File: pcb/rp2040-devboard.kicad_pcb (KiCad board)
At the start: 2 copper layers, 37.8 x 62.5 mm, 35 parts, among them J201 USB_C_Receptacle_USB2.0_16P, J601 Conn_01x20, J602 Conn_01x20, J603 Conn_01x03, SW401 SW_Push, SW501 SW_Push, U301 TC1017-xLT, U401 RP2040, U501 W25Q128JVS, Y401 ABM8-272-T3

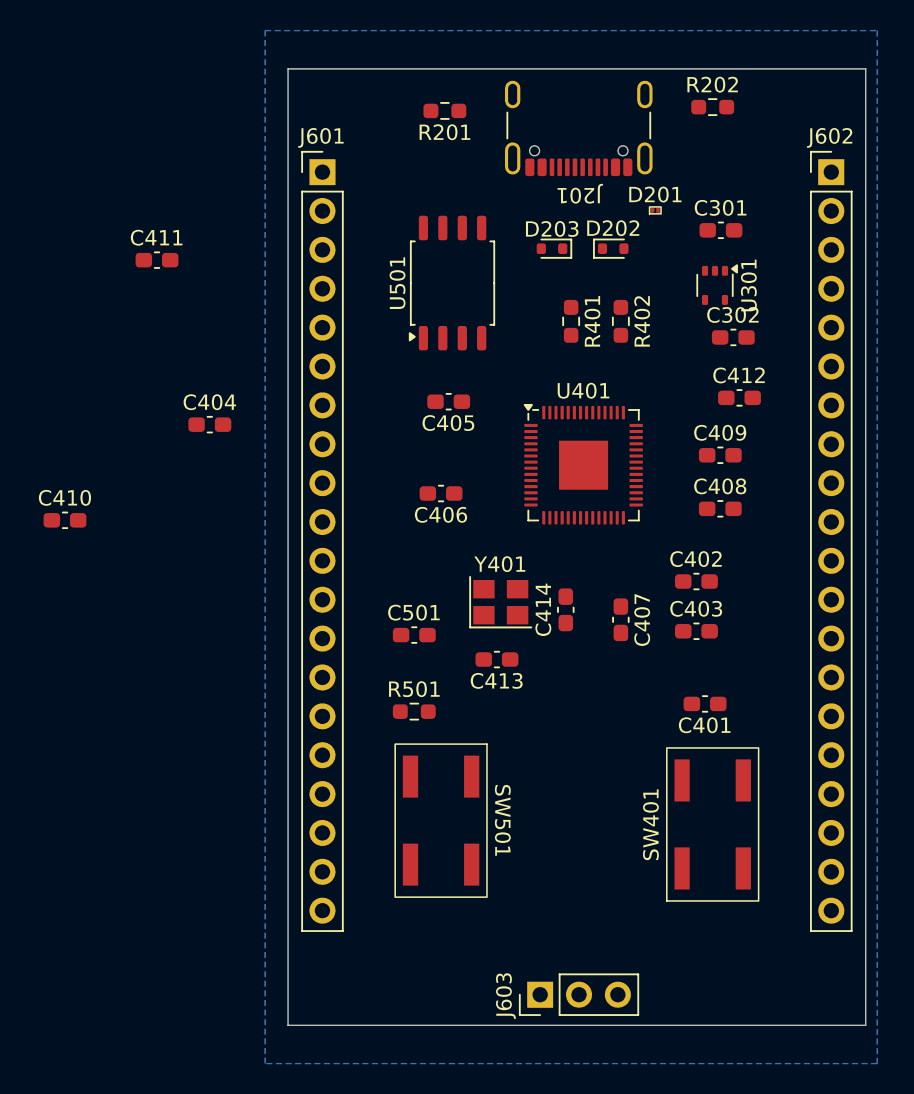
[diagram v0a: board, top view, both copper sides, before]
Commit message: wip pcb placement
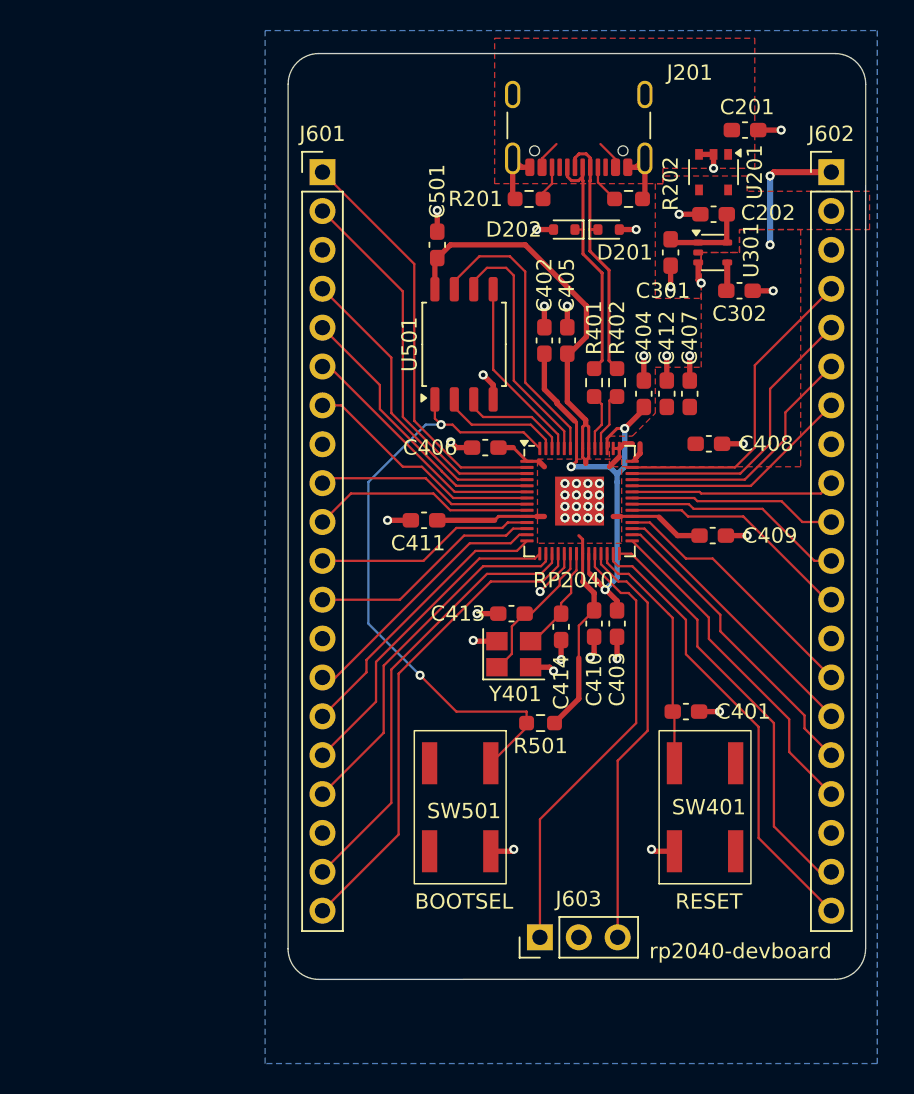
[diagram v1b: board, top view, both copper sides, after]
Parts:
- removed the D201 at (163.0, 56.8)
- added C201: 1u, Capacitor_SMD:C_0603_1608Metric_Pad1.08x0.95mm_HandSolder, F.Cu at (168.9, 51.5)
- added C202: 1u, Capacitor_SMD:C_0603_1608Metric_Pad1.08x0.95mm_HandSolder, F.Cu at (166.8, 57.0)
- added U201: NCP360SN, Package_SO:TSOP-5_1.65x3.05mm_P0.95mm, F.Cu at (166.8, 54.2)
- moved C410 35.2 mm to (159.0, 83.8), turned to -90 degrees
- moved C404 28.4 mm to (162.2, 68.7), turned to 90 degrees
- moved C501 25.5 mm to (148.8, 59.0), turned to 90 degrees
- moved C411 24.4 mm to (147.9, 77.0), turned to 180 degrees
- moved C402 18.6 mm to (155.8, 65.2), turned to 90 degrees
- moved C407 15.4 mm to (165.2, 68.7), turned to 90 degrees
- moved C405 8.72 mm to (157.2, 65.2), turned to 90 degrees
- moved R501 8.28 mm to (155.5, 90.2), turned to 180 degrees
- moved R202 8.14 mm to (161.2, 56.0)
- moved R201 7.96 mm to (154.8, 56.0)
- moved C409 5.27 mm to (166.8, 78.0)
- moved C403 5.21 mm to (160.5, 83.8), turned to -90 degrees
- moved C412 4.76 mm to (163.8, 68.7), turned to 90 degrees
- moved C408 4.32 mm to (166.5, 72.0)
- moved R401 4.27 mm to (159.0, 68.0)
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- renumbered D202 to D201, D203 to D202
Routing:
- net +3V3: track 0.00 -> 73.1 mm, vias 0 -> 2
- net GND: track 0.00 -> 52.4 mm, vias 0 -> 45
- net /Flash/QSPI_SS: track 0.00 -> 42.0 mm, vias 0 -> 2
- net /IO/GPIO15: track 0.00 -> 31.7 mm
- net +1V1: track 0.00 -> 31.1 mm, vias 0 -> 3
- net /IO/GPIO16: track 0.00 -> 29.8 mm
- net /IO/SWCLK: track 0.00 -> 29.1 mm
- net /IO/GPIO14: track 0.00 -> 29.1 mm
- net /IO/SWD: track 0.00 -> 27.5 mm
- net /IO/GPIO17: track 0.00 -> 27.4 mm
- net /IO/GPIO0: track 0.00 -> 27.4 mm
- net /IO/GPIO1: track 0.00 -> 25.3 mm
- net /IO/GPIO13: track 0.00 -> 24.0 mm
- net /IO/GPIO18: track 0.00 -> 21.9 mm
- net /IO/GPIO12: track 0.00 -> 21.2 mm
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- added copper zone on F.Cu, net +3V3
- added copper zone on F.Cu, net +5V
- added copper zone on F.Cu, net VBUS
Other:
- board size 37.8 x 62.5 mm -> 37.8 x 60.5 mm
- board text added: "3V3"
- board text added: "5V"
- board text added: "BOOTSEL"
- board text added: "GND"
- board text added: "GPIO0"
- board text added: "GPIO1"
- board text added: "GPIO10"
- board text added: "GPIO11"
- board text added: "GPIO12"
- board text added: "GPIO13"
- board text added: "GPIO14"
- board text added: "GPIO15"
- board text added: "GPIO16"
- board text added: "GPIO17"
- board text added: "GPIO18"
- board text added: "GPIO19"
- board text added: "GPIO2"
- board text added: "GPIO20"
- board text added: "GPIO21"
- board text added: "GPIO22"
- board text added: "GPIO23"
- board text added: "GPIO24"
- board text added: "GPIO25"
- board text added: "GPIO26"
- board text added: "GPIO27"
- board text added: "GPIO28"
- board text added: "GPIO29"
- board text added: "GPIO3"
- board text added: "GPIO4"
- board text added: "GPIO5"
- board text added: "GPIO6"
- board text added: "GPIO7"
- board text added: "GPIO8"
- board text added: "GPIO9"
- board text added: "RESET"
- board text added: "RP2040"
- board text added: "SWCLK"
- board text added: "SWD"
- board text added: "rp2040-devboard"
